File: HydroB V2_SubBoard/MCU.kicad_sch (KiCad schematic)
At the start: 36 parts, among them J4 Conn_01x04_Pin, J5 Conn_01x02_Pin, J7 Conn_01x02_Pin, Q6 S8050, Q7 S8050, Q8 S8050, SW1 SW_Push, U1 STM32F103C8Tx, Y1 8Mhz

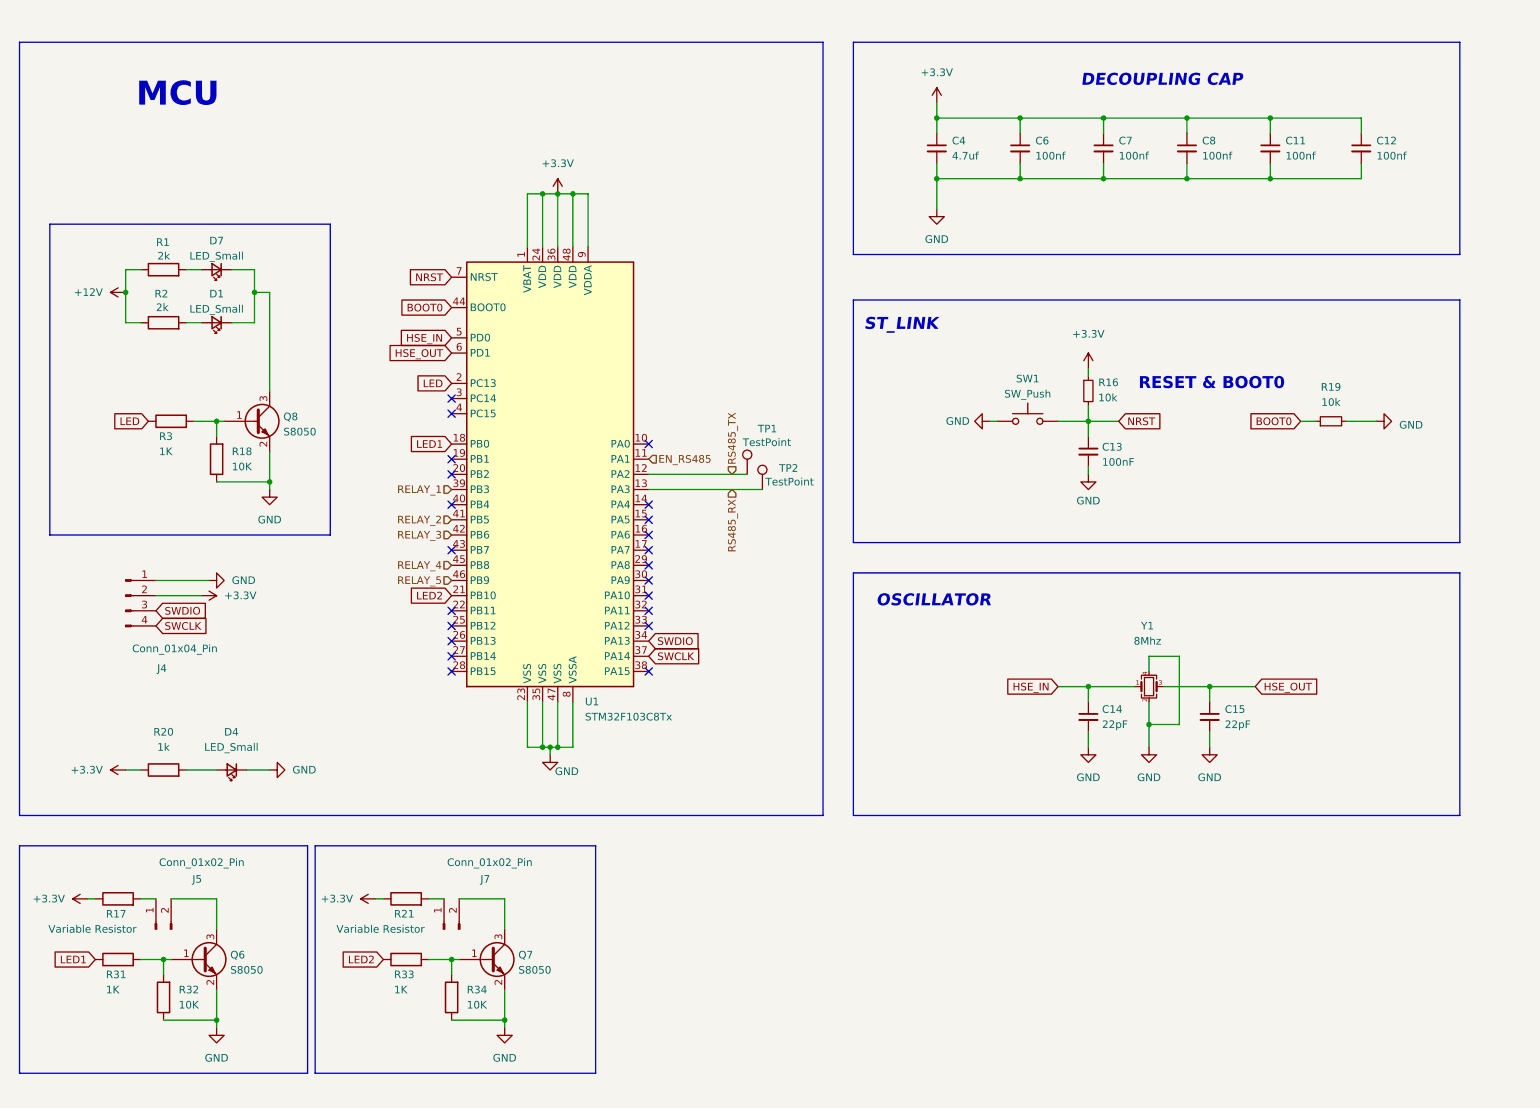
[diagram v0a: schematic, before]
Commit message: PCB update
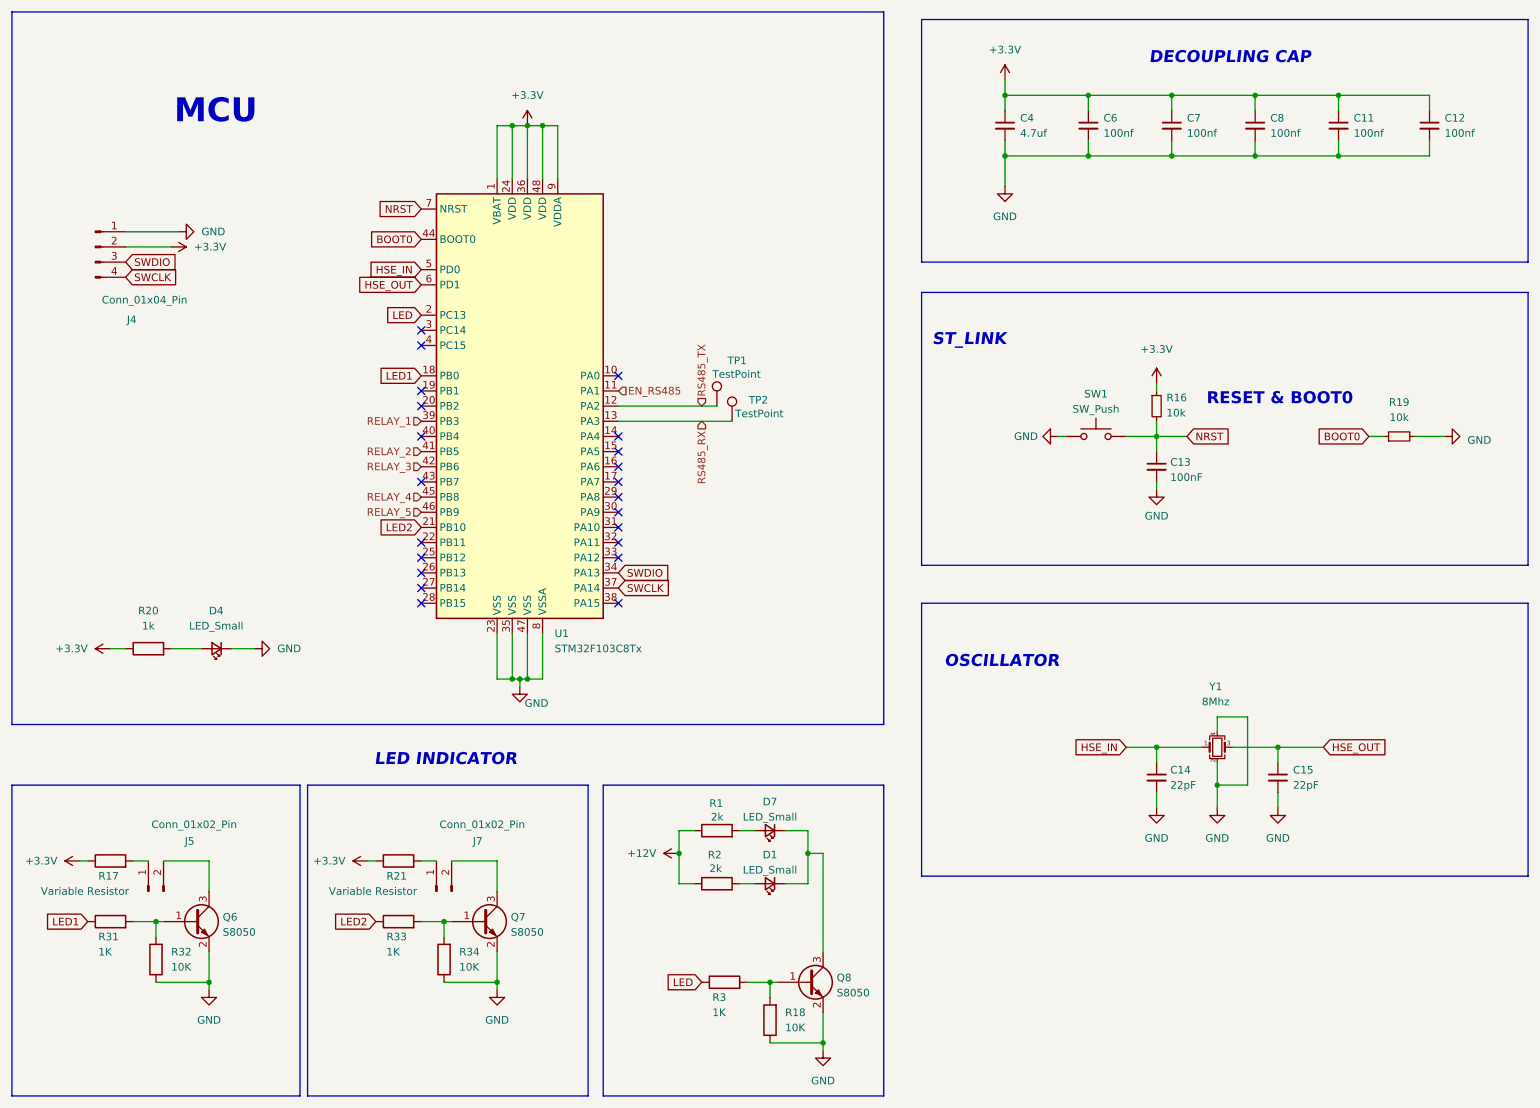
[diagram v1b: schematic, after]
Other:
- note added: "LED INDICATOR"
- moved on the sheet: C11, C12, C13, C14, C15, C4, C6, C7, C8, D1, D4, D7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
